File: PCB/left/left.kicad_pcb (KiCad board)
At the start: 2 copper layers, 3.4 x 3 mm, 49 parts, among them SW1 SW_Push_45deg, SW10 SW_Push_45deg, SW11 SW_Push_45deg, SW12 SW_Push_45deg, SW13 SW_Push_45deg, SW14 SW_Push_45deg, SW15 SW_Push_45deg, SW16 SW_Push_45deg, SW17 SW_Push_45deg, SW18 SW_Push_45deg, SW19 SW_Push, SW2 SW_Push_45deg, SW3 SW_Push_45deg, SW4 SW_Push_45deg, SW5 SW_Push_45deg, SW6 SW_Push_45deg, SW7 SW_Push_45deg, SW8 SW_Push_45deg, SW9 SW_Push_45deg, U1 COM-09032, U2 TRRS

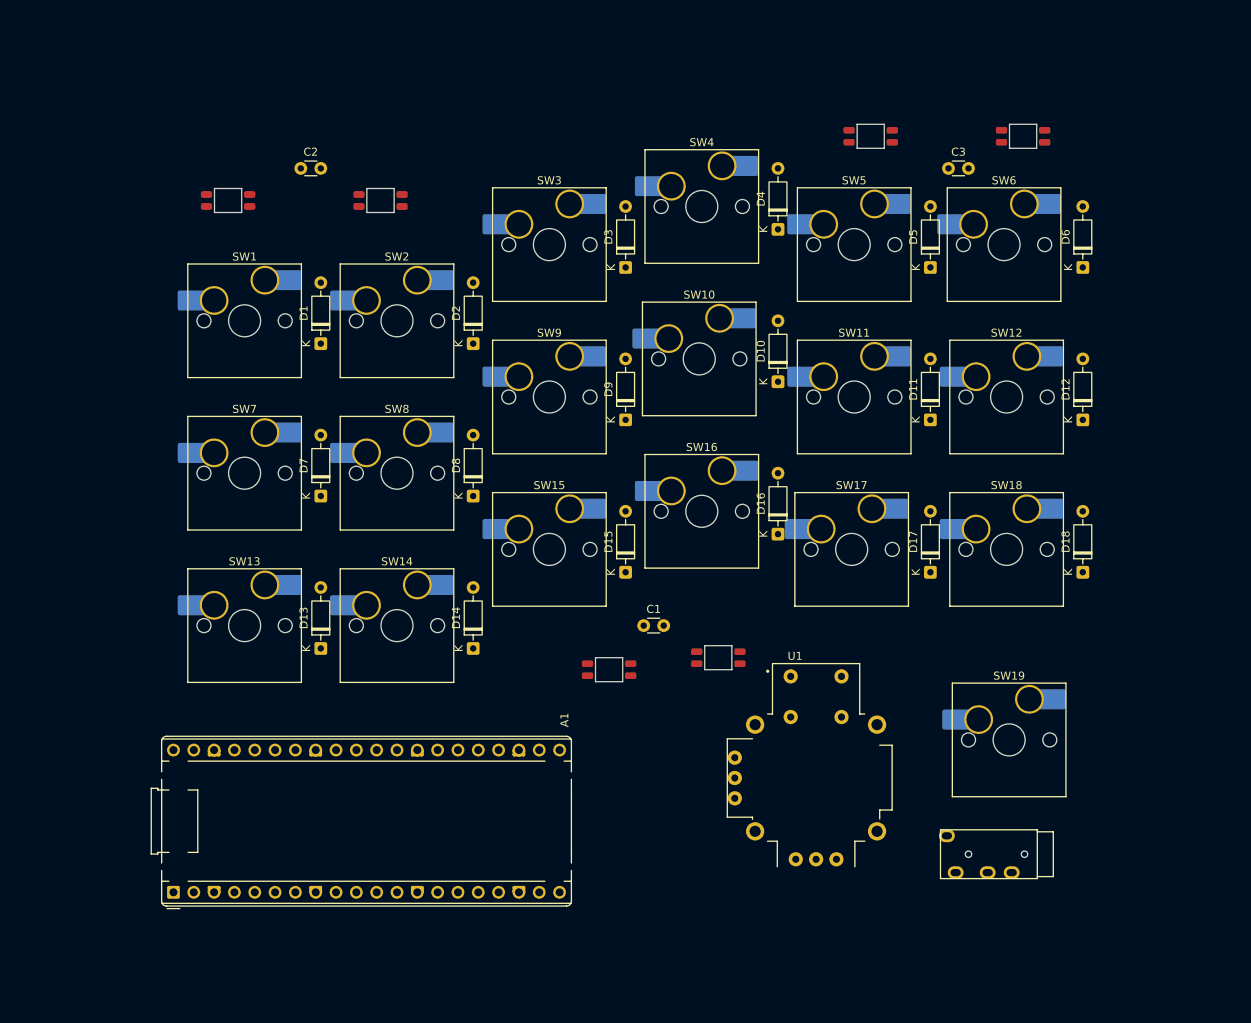
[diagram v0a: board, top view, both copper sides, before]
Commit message: [ JUN 9 // ROUTING ]
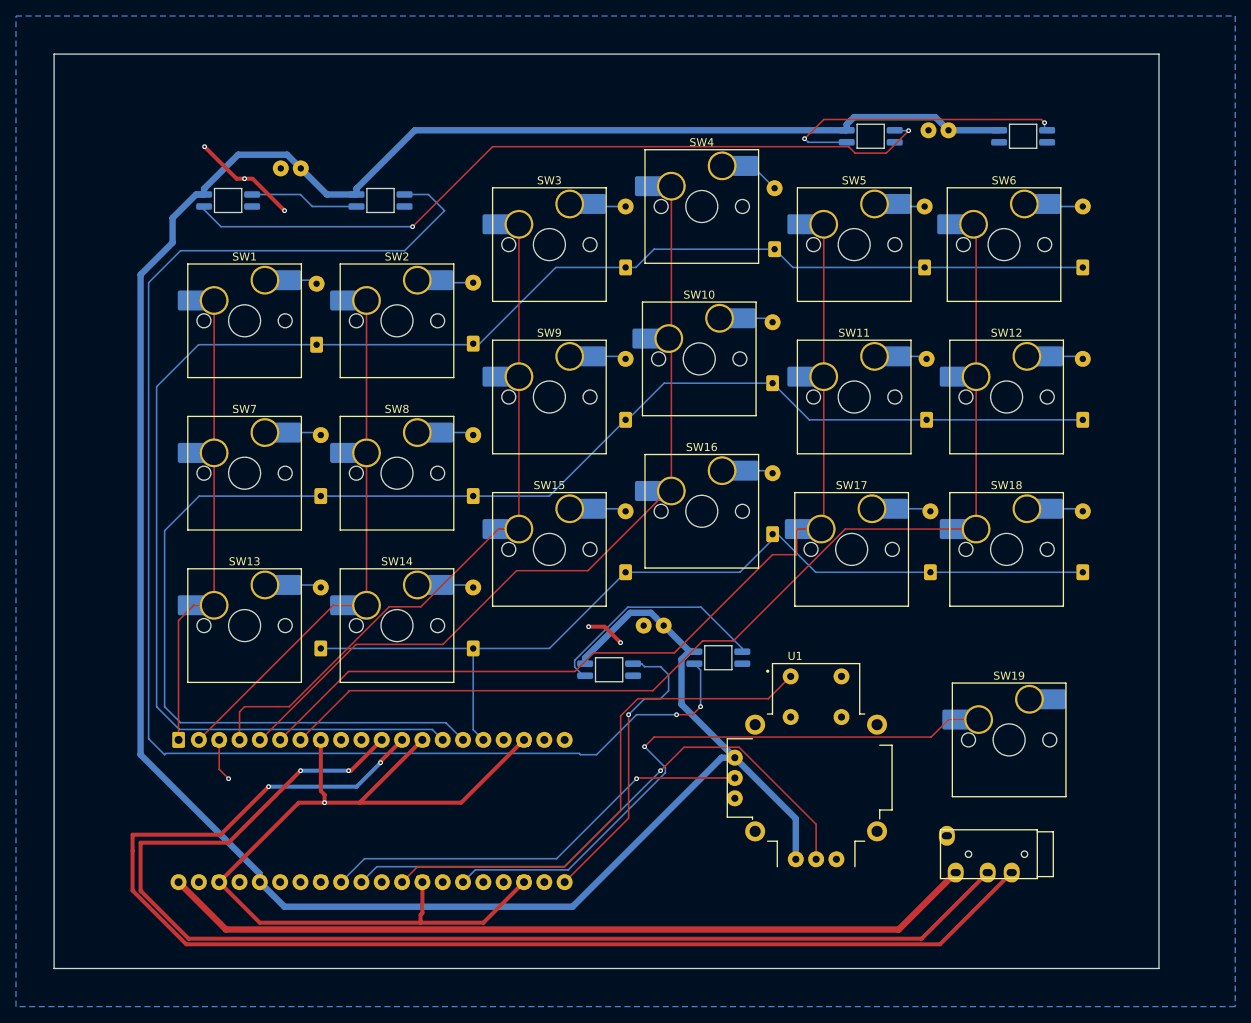
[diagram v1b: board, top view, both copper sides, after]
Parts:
- A1, C1, C2, C3, D19, D20, D21, D22, D23, D24: moved to B.Cu
- D1, D10, D11, D12, D13, D14, D15, D16, D17, D18, D2, D3, D4, D5, D6, D7, D8, D9: footprint Diode_THT:D_DO-35_SOD27_P7.62mm_Horizontal -> ScottoKeebs_Miscellaneous:D_DO-35_SOD27_P7.62mm_Horizontal-bigpads; moved to B.Cu
- moved A1 19.1 mm to (34.3, 109.5), turned to -90 degrees
- moved C3 4.76 mm to (130.5, 33.3), turned to 180 degrees
- moved D4 2.51 mm to (108.8, 48.2)
- moved C1 2.50 mm to (94.9, 95.2), turned to 180 degrees
- moved D5 0.73 mm to (127.5, 50.5)
- moved D10 0.70 mm to (108.5, 64.9)
- moved D16 0.67 mm to (108.5, 83.8)
- moved D1 0.54 mm to (51.5, 60.1)
- moved D11 0.48 mm to (127.8, 69.5)
- turned C2 to 180 degrees
- turned D19 to 180 degrees
- turned D20 to 180 degrees
- turned D21 to 180 degrees
- turned D22 to 180 degrees
- turned D23 to 180 degrees
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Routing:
- net +3V3: track 0.00 -> 326.0 mm
- net ROW0: track 0.00 -> 201.3 mm
- net ROW1: track 0.00 -> 185.3 mm
- net Net-(D20-DOUT): track 0.00 -> 182.6 mm, vias 0 -> 2
- net RX: track 0.00 -> 162.1 mm, vias 0 -> 2
- net TX: track 0.00 -> 153.3 mm, vias 0 -> 2
- net GND: track 0.00 -> 135.6 mm, vias 0 -> 7
- net COL5: track 0.00 -> 133.7 mm
- net COL4: track 0.00 -> 118.5 mm
- net ROW2: track 0.00 -> 115.1 mm
- net Net-(A1-VBUS): track 0.00 -> 102.5 mm
- net COL3: track 0.00 -> 102.4 mm
- net Net-(D22-DOUT): track 0.00 -> 96.7 mm, vias 0 -> 2
- net COL2: track 0.00 -> 86.0 mm
- net Net-(A1-GPIO20): track 0.00 -> 78.5 mm, vias 0 -> 1
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- added copper zone on B.Cu, net GND
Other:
- board size 3.4 x 3 mm -> 138.1 x 114.3 mm
